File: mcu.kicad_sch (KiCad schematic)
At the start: 124 parts, among them Q1 NMOS, Q2 NMOS, SW1 SW_Push, U1 PIC32CK1025GC01100-I/4SB, Y1 Crystal, Y2 Crystal

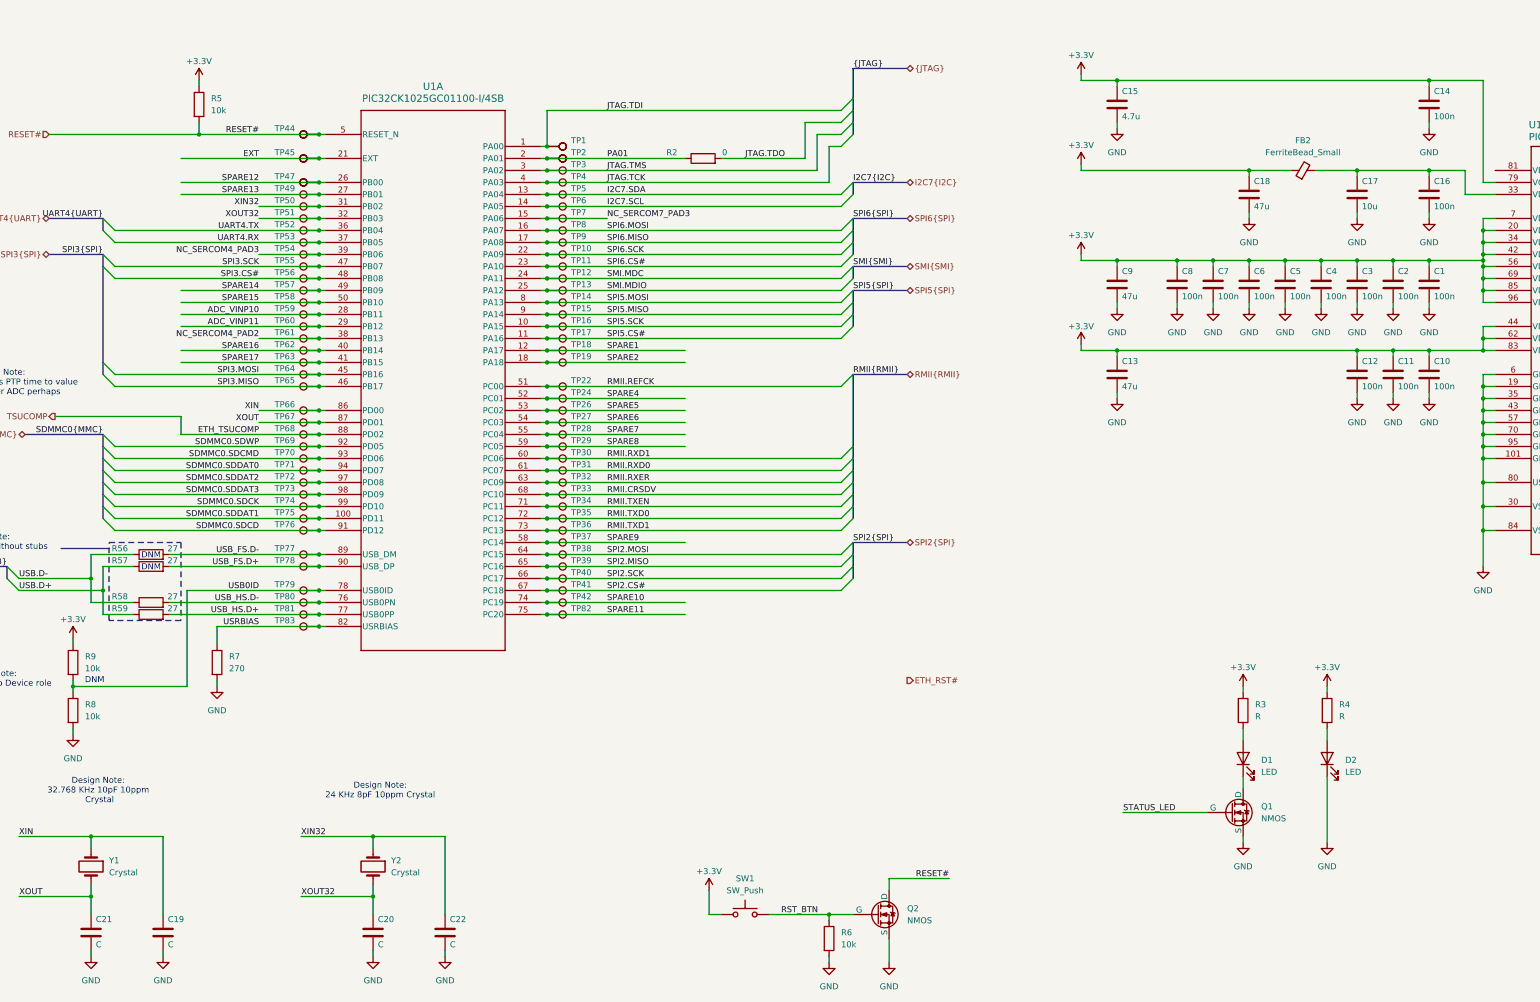
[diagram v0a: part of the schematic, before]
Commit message: did stuff
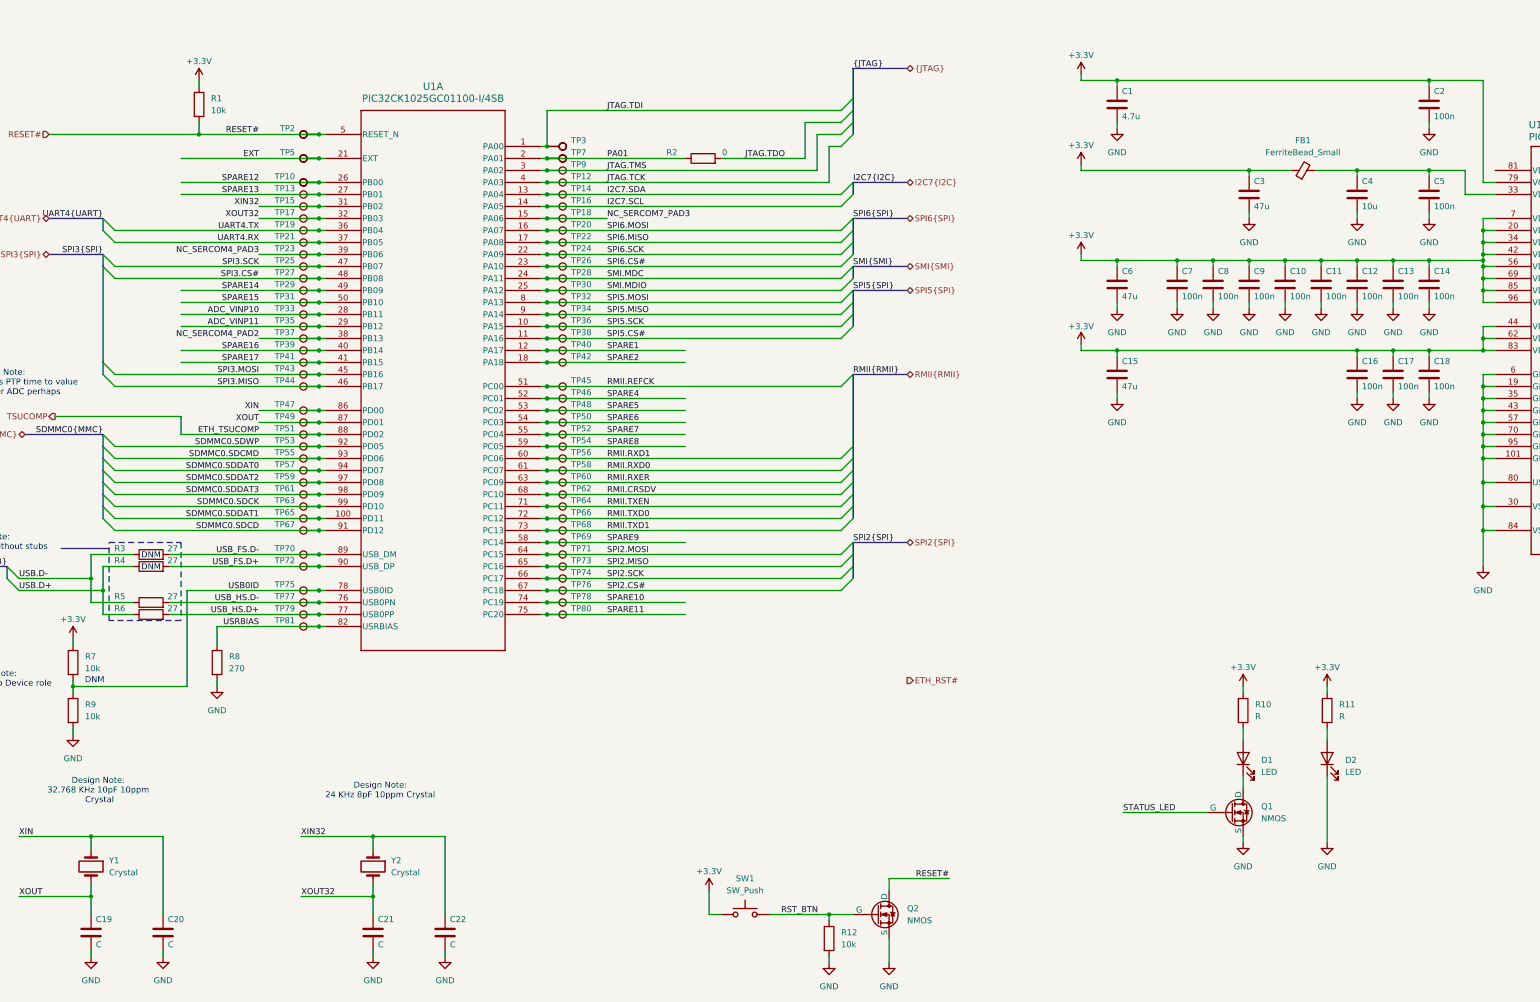
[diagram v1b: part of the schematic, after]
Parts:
- renumbered C15 to C1, C5 to C10, C4 to C11, C3 to C12, C2 to C13, C1 to C14, C13 to C15, C12 to C16, C11 to C17, C10 to C18, C21 to C19, C14 to C2, C19 to C20, C20 to C21, C18 to C3, C17 to C4, C16 to C5, C9 to C6, C8 to C7, C7 to C8, C6 to C9, FB2 to FB1, R5 to R1, R3 to R10, R4 to R11, R6 to R12, R56 to R3, R57 to R4, R58 to R5, R59 to R6, R9 to R7, R7 to R8, R8 to R9, TP43 to TP1, TP47 to TP10, TP48 to TP11, TP4 to TP12, TP49 to TP13, TP5 to TP14, TP50 to TP15, TP6 to TP16, TP51 to TP17, TP7 to TP18, TP52 to TP19, TP44 to TP2, TP8 to TP20, TP53 to TP21, TP9 to TP22, TP54 to TP23, TP10 to TP24, TP55 to TP25, TP11 to TP26, TP56 to TP27, TP12 to TP28, TP57 to TP29, TP1 to TP3, TP13 to TP30, TP58 to TP31, TP14 to TP32, TP59 to TP33, TP15 to TP34, TP60 to TP35, TP16 to TP36, TP61 to TP37, TP17 to TP38, TP62 to TP39, TP20 to TP4, TP18 to TP40, TP63 to TP41, TP19 to TP42, TP64 to TP43, TP65 to TP44, TP22 to TP45, TP24 to TP46, TP66 to TP47, TP26 to TP48, TP67 to TP49, TP45 to TP5, TP27 to TP50, TP68 to TP51, TP28 to TP52, TP69 to TP53, TP29 to TP54, TP70 to TP55, TP30 to TP56, TP71 to TP57, TP31 to TP58, TP72 to TP59, TP46 to TP6, TP32 to TP60, TP73 to TP61, TP33 to TP62, TP74 to TP63, TP34 to TP64, TP75 to TP65, TP35 to TP66, TP76 to TP67, TP36 to TP68, TP37 to TP69, TP2 to TP7, TP77 to TP70, TP38 to TP71, TP78 to TP72, TP39 to TP73, TP40 to TP74, TP79 to TP75, TP41 to TP76, TP80 to TP77, TP42 to TP78, TP81 to TP79, TP21 to TP8, TP82 to TP80, TP83 to TP81, TP3 to TP9
